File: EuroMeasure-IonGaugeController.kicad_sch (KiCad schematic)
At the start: 25 parts, among them J1 Conn_02x05_Odd_Even, U1 ADS131M04-WQFN, X1 8.192MHz

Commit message: Final 1.0.0 version
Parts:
- J1: MPN (none) -> NO_MPN
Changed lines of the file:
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@@
+      (effects (font (size 1.27 1.27)) hide)
+    )
+    (property "MPN" "NO_MPN" (at 125.73 138.43 0)
       (effects (font (size 1.27 1.27)) hide)
     )

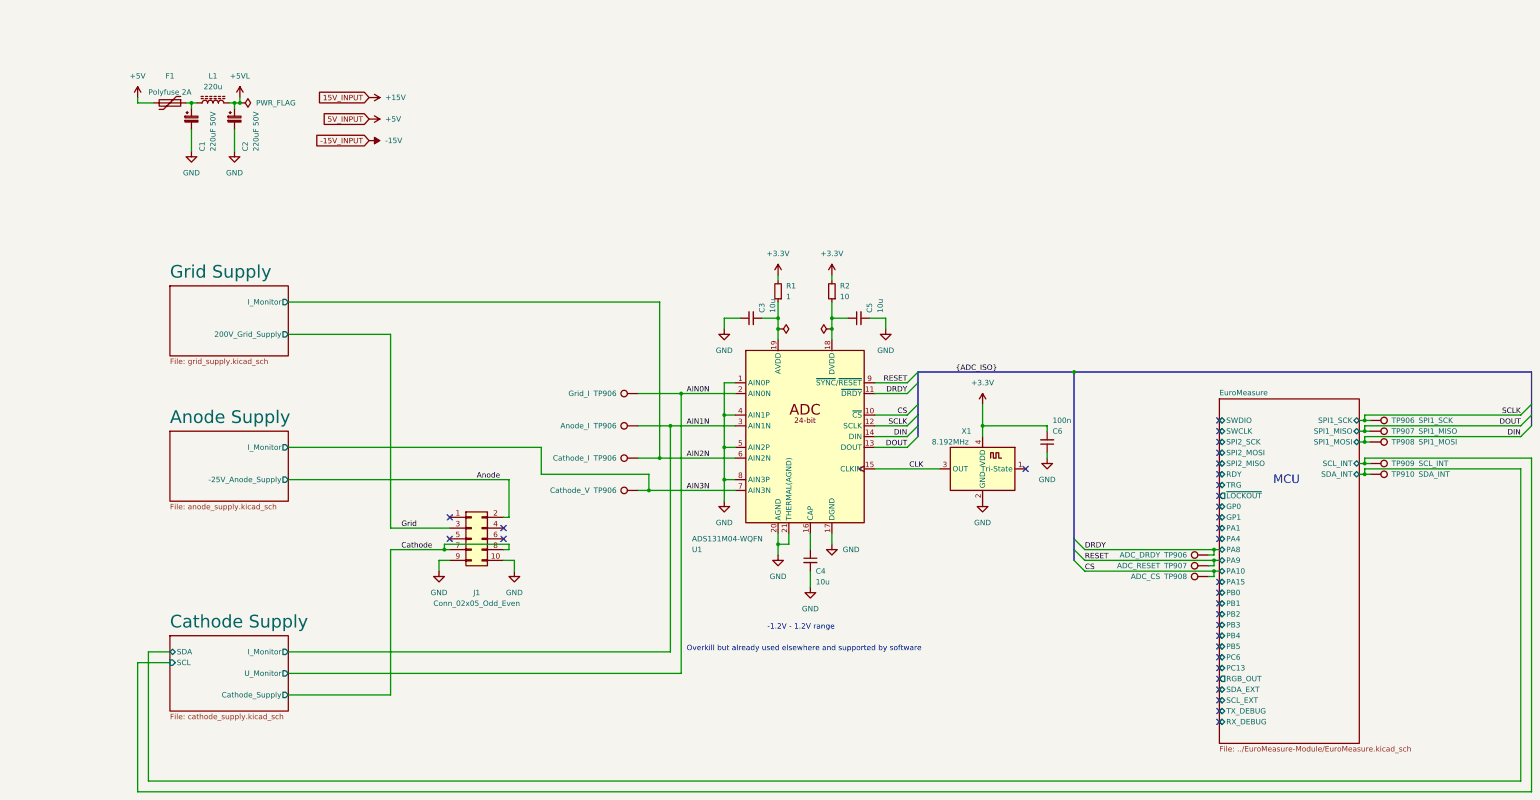
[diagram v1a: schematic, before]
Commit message: Revision 1.1.0. DRC clean
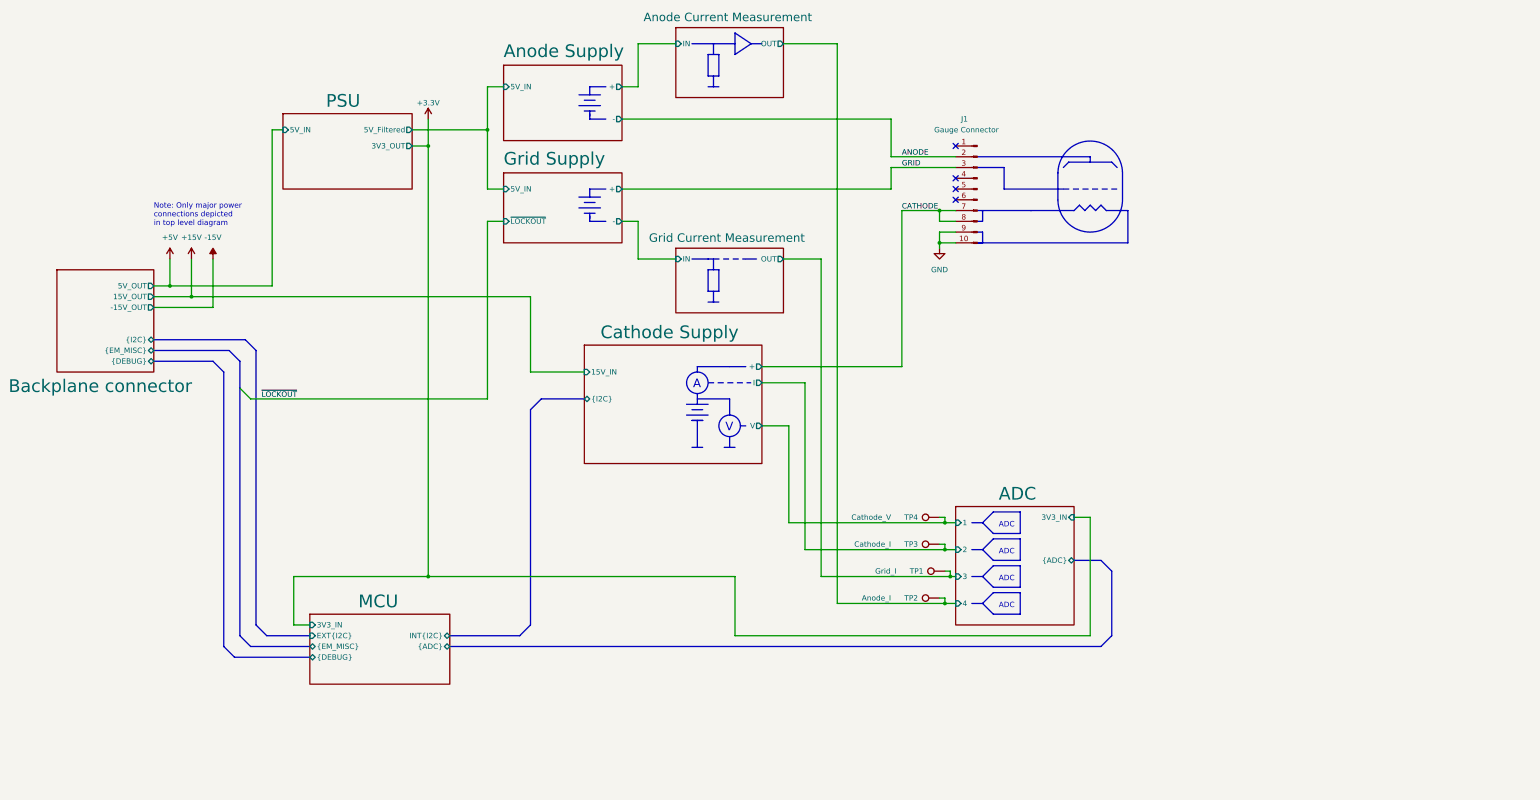
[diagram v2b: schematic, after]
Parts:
- removed C1, C2: 220uF 50V, Capacitor_SMD:CP_Elec_6.3x7.7, symbol MEMS_Passive:C_Elec-220uf-50V
- removed C3, C4, C5: 10u, Capacitor_SMD:C_0805_2012Metric_Pad1.18x1.45mm_HandSolder, symbol Device:C_Small
- removed C6: 100n, Capacitor_SMD:C_0805_2012Metric_Pad1.18x1.45mm_HandSolder, symbol Device:C_Small
- removed F1: Polyfuse 2A, MEMS_Passive:Fuse_Littlefuse_3425L, symbol MEMS_Protection:Polyfuse-2A-60V-3425L200/60MR
- removed J1: Conn_02x05_Odd_Even, Connector_IDC:IDC-Header_2x05_P2.54mm_Vertical, symbol Connector_Generic:Conn_02x05_Odd_Even
- removed L1: 220u, Inductor_SMD:L_12x12mm_H8mm, symbol MEMS_Passive:L_220u_10x10
- removed R1: 1, Resistor_SMD:R_0805_2012Metric_Pad1.20x1.40mm_HandSolder, symbol Device:R_Small
- removed R2: 10, Resistor_SMD:R_0805_2012Metric_Pad1.20x1.40mm_HandSolder, symbol Device:R_Small
- removed TP906: ADC_DRDY, MEMS_Custom:TestPoint_Pad_D1.0mm, symbol Connector:TestPoint
- removed TP906: Anode_I, MEMS_Custom:TestPoint_Pad_D1.0mm, symbol Connector:TestPoint
- removed TP906: Grid_I, MEMS_Custom:TestPoint_Pad_D1.0mm, symbol Connector:TestPoint
- removed TP906: Cathode_I, MEMS_Custom:TestPoint_Pad_D1.0mm, symbol Connector:TestPoint
- removed TP906: SPI1_SCK, MEMS_Custom:TestPoint_Pad_D1.0mm, symbol Connector:TestPoint
- removed TP906: Cathode_V, MEMS_Custom:TestPoint_Pad_D1.0mm, symbol Connector:TestPoint
- removed TP907: ADC_RESET, MEMS_Custom:TestPoint_Pad_D1.0mm, symbol Connector:TestPoint
- removed TP907: SPI1_MISO, MEMS_Custom:TestPoint_Pad_D1.0mm, symbol Connector:TestPoint
- removed TP908: SPI1_MOSI, MEMS_Custom:TestPoint_Pad_D1.0mm, symbol Connector:TestPoint
- removed TP908: ADC_CS, MEMS_Custom:TestPoint_Pad_D1.0mm, symbol Connector:TestPoint
- removed TP909: SCL_INT, MEMS_Custom:TestPoint_Pad_D1.0mm, symbol Connector:TestPoint
- removed TP910: SDA_INT, MEMS_Custom:TestPoint_Pad_D1.0mm, symbol Connector:TestPoint
- removed U1: ADS131M04-WQFN, Package_DFN_QFN:WQFN-20-1EP_3x3mm_P0.4mm_EP1.7x1.7mm, symbol MEMS_IC:ADS131M04-WQFN
- removed X1: 8.192MHz, Oscillator:Oscillator_SMD_ECS_2520MV-xxx-xx-4Pin_2.5x2.0mm, symbol MEMS_IC:ECS-2520MVLC-081.92-CN-TR_oscillator_8.192MHZ
- added J1: Gauge Connector, Connector_IDC:IDC-Header_2x05_P2.54mm_Horizontal, symbol Connector:Conn_01x10_Pin
- added TP1: Grid_I, MEMS_Custom:TestPoint_Pad_D1.0mm, symbol Connector:TestPoint
- added TP2: Anode_I, MEMS_Custom:TestPoint_Pad_D1.0mm, symbol Connector:TestPoint
- added TP3: Cathode_I, MEMS_Custom:TestPoint_Pad_D1.0mm, symbol Connector:TestPoint
- added TP4: Cathode_V, MEMS_Custom:TestPoint_Pad_D1.0mm, symbol Connector:TestPoint
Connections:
- net GND: now also J1.10 (Pin_10), J1.9 (Pin_9)
- new net ADC/1: TP4.1
- new net ADC/2: TP3.1
- new net ADC/3: TP1.1
- new net ADC/4: TP2.1
- new net ANODE: J1.2 (Pin_2)
- new net CATHODE: J1.7 (Pin_7), J1.8 (Pin_8)
- new net GRID: J1.3 (Pin_3)
- no-connect marks 31 -> 4
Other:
- sheet EuroMeasure renamed MCU
- added sheet ADC (adc.kicad_sch)
- added sheet Anode Current Measurement (anode_ammeter.kicad_sch)
- added sheet Backplane connector (backplane_connector.kicad_sch)
- added sheet Grid Current Measurement (grid_current_measurement.kicad_sch)
- added sheet PSU (psu.kicad_sch)
- sheet Anode Supply ports: added +, -, 5V_IN; removed -25V_Anode_Supply, I_Monitor
- sheet Cathode Supply ports: added +, 15V_IN, I, V, {I2C}; removed Cathode_Supply, I_Monitor, SCL, SDA, U_Monitor
- sheet Grid Supply ports: added +, -, 5V_IN, ~{LOCKOUT}; removed 200V_Grid_Supply, I_Monitor
- sheet MCU: file ../EuroMeasure-Module/EuroMeasure.kicad_sch -> MCU.kicad_sch
- sheet MCU ports: added 3V3_IN, EXT{I2C}, INT{I2C}, {ADC}, {DEBUG}, {EM_MISC}; removed GP0, GP1, PA1, PA10, PA15, PA4, PA8, PA9, PB0, PB1, PB2, PB3, PB4, PB5, PC13, PC6, RDY, RGB_OUT, RX_DEBUG, SCL_EXT, SCL_INT, SDA_EXT, SDA_INT, SPI1_MISO, SPI1_MOSI, SPI1_SCK, SPI2_MISO, SPI2_MOSI, SPI2_SCK, SWCLK, SWDIO, TRG, TX_DEBUG, ~{LOCKOUT}
- note added: "A"
- note added: "ADC"
- note added: "Note: Only major power connections depicted in top level diagram"
- note added: "V"
- note removed: "-1.2V - 1.2V range"
- note removed: "MCU"
- note removed: "Overkill but already used elsewhere and supported by software"
